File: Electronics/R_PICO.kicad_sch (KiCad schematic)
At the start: 14 parts, among them U1 R-785.0-0.5, U2 VL53L0CXV0DH1, U3 VL53L0CXV0DH1, U4 VL53L0CXV0DH1, U5 VL53L0CXV0DH1, U6 TB6612FNG

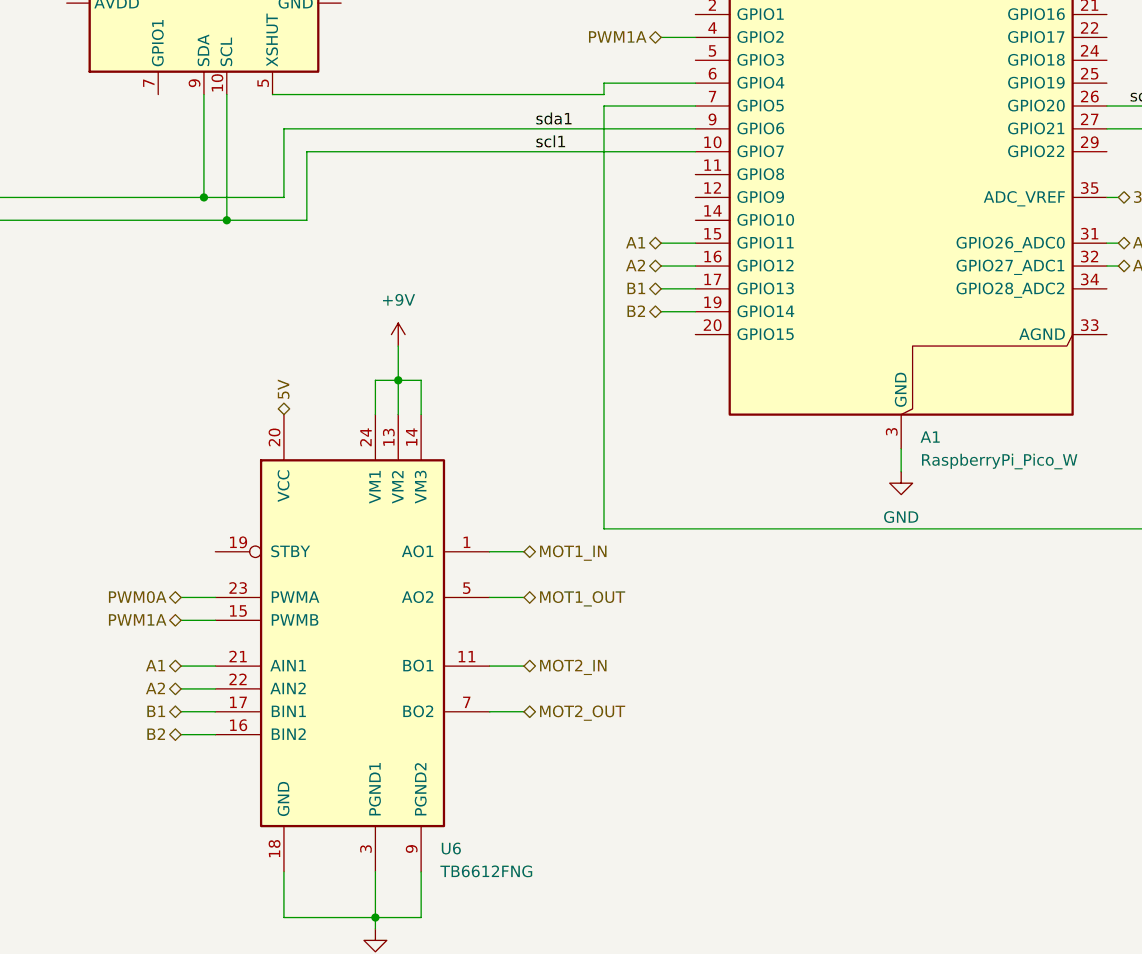
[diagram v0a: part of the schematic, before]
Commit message: added starter scheme
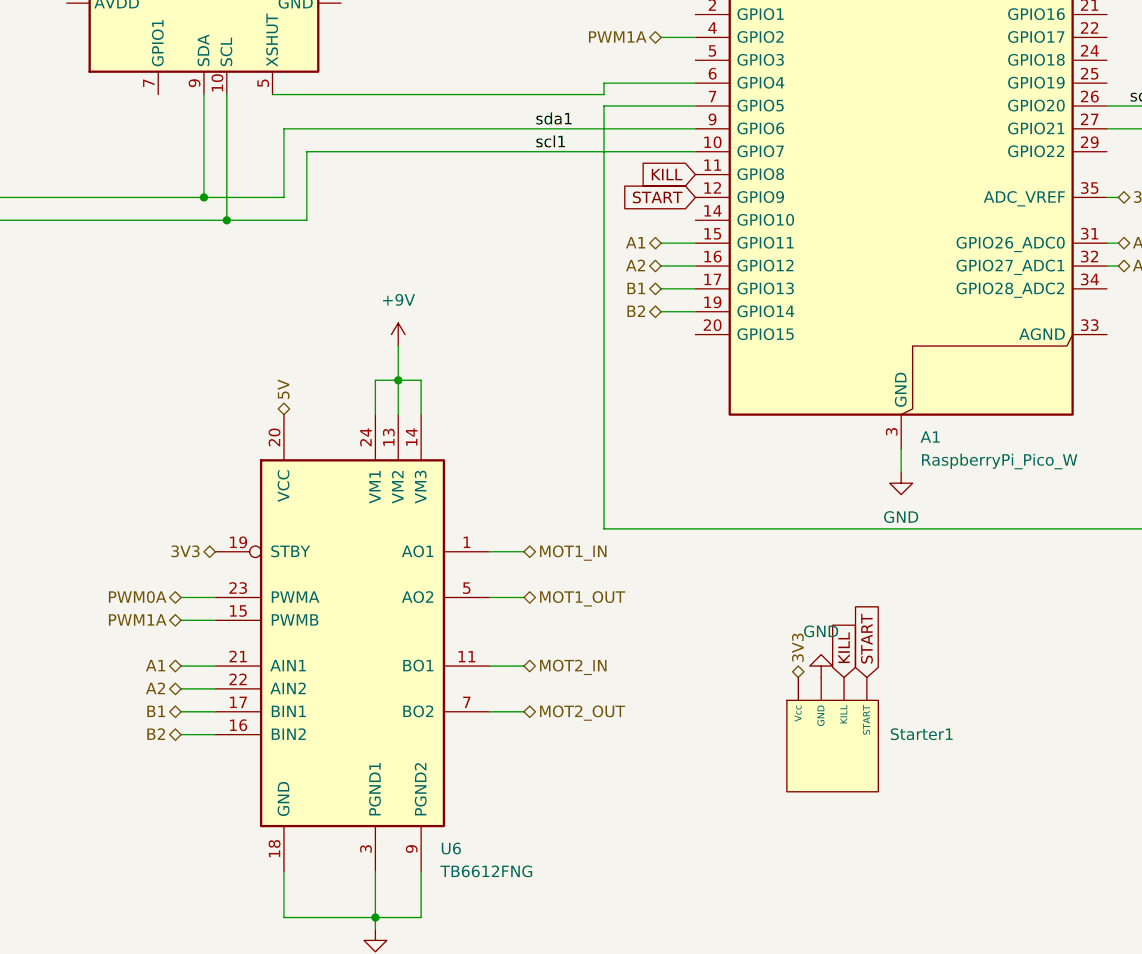
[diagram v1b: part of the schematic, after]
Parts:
- added Starter1: ~, symbol Own:Starter
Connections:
- net 3V3: now also U6.19 (STBY), Starter1. (START)
- net GND: now also Starter1. (START)
- net KILL: now reaches A1.11 (GPIO8)
- net KILL: now also Starter1. (START)
- net START: now reaches A1.12 (GPIO9)
- net START: now also Starter1. (START)
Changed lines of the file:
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@@
+		)
+	)
+	(global_label "KILL"
+		(shape input)
+		(at 146.05 130.81 90)
+		(fields_autoplaced yes)
+		(effects
+			(font
+				(size 1.27 1.27)
+			)
+			(justify left)
+		)
+		(property "Intersheetrefs" "${INTERSHEET_REFS}"
+			(at 146.05 123.8938 90)
+			(effects
+				(font
+					(size 1.27 1.27)
+				)
+				(justify left)
+				(hide yes)
+			)
+		)
+	)
+	(global_label "START"
+		(shape input)
+		(at 129.54 77.47 180)
+		(fields_autoplaced yes)
+		(effects
+			(font
+				(size 1.27 1.27)
+			)
+			(justify right)
+		)
+		(property "Intersheetrefs" "${INTERSHEET_REFS}"
+			(at 121.0515 77.47 0)
+			(effects
+				(font
+					(size 1.27 1.27)
+				)
+				(justify right)
+				(hide yes)
+			)
+		)
+	)
+	(global_label "KILL"
+		(shape input)
+		(at 129.54 74.93 180)
+		(fields_autoplaced yes)
+		(effects
+			(font
+				(size 1.27 1.27)
+			)
+			(justify right)
+		)
+		(property "Intersheetrefs" "${INTERSHEET_REFS}"
+			(at 122.6238 74.93 0)
+			(effects
+				(font
+					(size 1.27 1.27)
+				)
+				(justify right)
+				(hide yes)
+			)
+		)
+	)
+	(global_label "START"
+		(shape input)
+		(at 148.59 130.81 90)
+		(fields_autoplaced yes)
+		(effects
+			(font
+				(size 1.27 1.27)
+			)
+			(justify left)
+		)
+		(property "Intersheetrefs" "${INTERSHEET_REFS}"
+			(at 148.59 122.3215 90)
+			(effects
+				(font
+					(size 1.27 1.27)
+				)
+				(justify left)
+				(hide yes)
+			)
 		)
 	)
@@
 		)
 	)
+	(hierarchical_label "3V3"
+		(shape bidirectional)
+		(at 76.2 116.84 180)
+		(effects
+			(font
+				(size 1.27 1.27)
+			)
+			(justify right)
+		)
+	)
 	(hierarchical_label "5V"
 		(shape bidirectional)
@@
 			)
 			(justify right)
+		)
+	)
+	(hierarchical_label "3V3"
+		(shape bidirectional)
+		(at 140.97 130.81 90)
+		(effects
+			(font
+				(size 1.27 1.27)
+			)
+			(justify left)
 		)
 	)
@@
 	)
 	(symbol
+		(lib_id "Own:Starter")
+		(at 143.51 128.27 0)
+		(unit 1)
+		(exclude_from_sim no)
+		(in_bom yes)
+		(on_board yes)
+		(dnp no)
+		(fields_autoplaced yes)
+		(property "Reference" "Starter1"
+			(at 151.13 137.1599 0)
+			(effects
+				(font
+					(size 1.27 1.27)
+				)
+				(justify left)
+			)
+		)
+		(property "Value" "~"
+			(at 151.13 139.6999 0)
+			(effects
+				(font
+					(size 1.27 1.27)
+				)
+				(justify left)
+			)
+		)
+		(property "Footprint" ""
+			(at 143.51 128.27 0)
+			(effects
+				(font
+					(size 1.27 1.27)
+				)
+				(hide yes)
+			)
+		)
+		(property "Datasheet" ""
+			(at 143.51 128.27 0)
+			(effects
+				(font
+					(size 1.27 1.27)
+				)
+				(hide yes)
+			)
+		)
+		(property "Description" ""
+			(at 143.51 128.27 0)
+			(effects
+				(font
+					(size 1.27 1.27)
+				)
+				(hide yes)
+			)
+		)
+		(pin ""
+		)
+		(pin ""
+		)
+		(pin ""
+		)
+		(pin ""
+		)
+		(instances
+			(project ""
+				(path "/8d834d26-b607-404e-affc-aead426ecb0a"
+					(reference "Starter1")
+					(unit 1)
+				)
+			)
+		)
+	)
+	(symbol
 		(lib_id "power:GND")
 		(at 240.03 142.24 0)
@@
 					(unit 1)
 				)
+			)
+		)
+	)
+	(symbol
+		(lib_id "power:GND")
+		(at 143.51 130.81 180)
+		(unit 1)
+		(exclude_from_sim no)
+		(in_bom yes)
+		(on_board yes)
+		(dnp no)
+		(fields_autoplaced yes)
+		(property "Reference" "#PWR012"
+			(at 143.51 124.46 0)
+			(effects
+				(font
+					(size 1.27 1.27)
+				)
+				(hide yes)
+			)
+		)
+		(property "Value" "GND"
+			(at 143.51 125.73 0)
+			(effects
+				(font
+					(size 1.27 1.27)
+				)
+			)
+		)
+		(property "Footprint" ""
+			(at 143.51 130.81 0)
+			(effects
+				(font
+					(size 1.27 1.27)
+				)
+				(hide yes)
+			)
+		)
+		(property "Datasheet" ""
+			(at 143.51 130.81 0)
+			(effects
+				(font
+					(size 1.27 1.27)
+				)
+				(hide yes)
+			)
+		)
+		(property "Description" "Power symbol creates a global label with name \"GND\" , ground"
+			(at 143.51 130.81 0)
+			(effects
+				(font
+					(size 1.27 1.27)
+				)
+				(hide yes)
+			)
+		)
+		(pin "1"
+		)
+		(instances
+			(project "R_PICO"
+				(path "/8d834d26-b607-404e-affc-aead426ecb0a"
+					(reference "#PWR012")
+					(unit 1)
+				)
